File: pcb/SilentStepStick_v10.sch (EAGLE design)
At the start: 30 parts, among them X1 PASSER-07, X2 PASSER-07

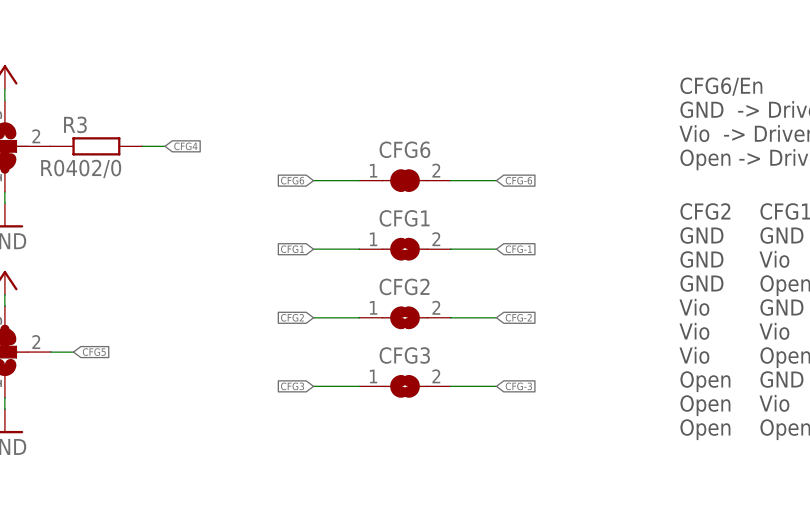
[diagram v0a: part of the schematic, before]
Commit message: updated layout and schematics
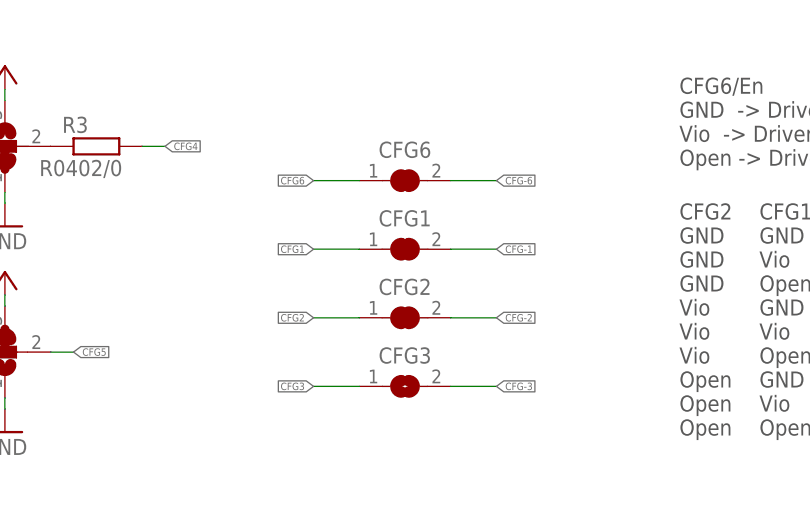
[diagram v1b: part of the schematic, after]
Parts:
- CFG1, CFG2, CFG3, CFG6: value JUMPER2-0201-NC -> JUMPER2-0201; device we-rcl:JUMPER2-0201-NC -> we-rcl:JUMPER2-0201
- CFG5: value JUMPER3-0201-NC -> JUMPER3-0201; device we-rcl:JUMPER3-0201-NC -> we-rcl:JUMPER3-0201
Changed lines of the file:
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@@
 <setting verticaltext="up"/>
 </settings>
-<grid distance="0.05" unitdist="inch" unit="inch" style="lines" multiple="1" display="yes" altdistance="0.025" altunitdist="inch" altunit="inch"/>
+<grid distance="0.1" unitdist="inch" unit="inch" style="lines" multiple="1" display="no" altdistance="0.01" altunitdist="inch" altunit="inch"/>
 <layers>
-<layer number="1" name="Top" color="4" fill="1" visible="no" active="no"/>
-<layer number="2" name="Route2" color="11" fill="1" visible="no" active="no"/>
-<layer number="3" name="Route3" color="4" fill="3" visible="no" active="no"/>
-<layer number="4" name="Route4" color="1" fill="4" visible="no" active="no"/>
-<layer number="5" name="Route5" color="4" fill="4" visible="no" active="no"/>
-<layer number="6" name="Route6" color="1" fill="8" visible="no" active="no"/>
-<layer number="7" name="Route7" color="4" fill="8" visible="no" active="no"/>
-<layer number="8" name="Route8" color="1" fill="2" visible="no" active="no"/>
-<layer number="9" name="Route9" color="4" fill="2" visible="no" active="no"/>
-<layer number="10" name="Route10" color="1" fill="7" visible="no" active="no"/>
-<layer number="11" name="Route11" color="4" fill="7" visible="no" active="no"/>
-<layer number="12" name="Route12" color="1" fill="5" visible="no" active="no"/>
-<layer number="13" name="Route13" color="4" fill="5" visible="no" active="no"/>
-<layer number="14" name="Route14" color="1" fill="6" visible="no" active="no"/>
-<layer number="15" name="Route15" color="13" fill="1" visible="no" active="no"/>
-<layer number="16" name="Bottom" color="1" fill="1" visible="no" active="no"/>
-<layer number="17" name="Pads" color="2" fill="1" visible="no" active="no"/>
-<layer number="18" name="Vias" color="2" fill="1" visible="no" active="no"/>
-<layer number="19" name="Unrouted" color="14" fill="1" visible="no" active="no"/>
-<layer number="20" name="Dimension" color="15" fill="1" visible="no" active="no"/>
-<layer number="21" name="tPlace" color="7" fill="1" visible="no" active="no"/>
-<layer number="22" name="bPlace" color="7" fill="1" visible="no" active="no"/>
-<layer number="23" name="tOrigins" color="15" fill="1" visible="no" active="no"/>
-<layer number="24" name="bOrigins" color="15" fill="1" visible="no" active="no"/>
-<layer number="25" name="tNames" color="7" fill="1" visible="no" active="no"/>
-<layer number="26" name="bNames" color="7" fill="1" visible="no" active="no"/>
-<layer number="27" name="tValues" color="7" fill="1" visible="no" active="no"/>
-<layer number="28" name="bValues" color="7" fill="1" visible="no" active="no"/>
+<layer number="1" name="Top" color="4" fill="1" visible="yes" active="no"/>
+<layer number="2" name="Route2" color="11" fill="1" visible="yes" active="no"/>
+<layer number="3" name="Route3" color="4" fill="3" visible="yes" active="no"/>
+<layer number="4" name="Route4" color="1" fill="4" visible="yes" active="no"/>
+<layer number="5" name="Route5" color="4" fill="4" visible="yes" active="no"/>
+<layer number="6" name="Route6" color="1" fill="8" visible="yes" active="no"/>
+<layer number="7" name="Route7" color="4" fill="8" visible="yes" active="no"/>
+<layer number="8" name="Route8" color="1" fill="2" visible="yes" active="no"/>
+<layer number="9" name="Route9" color="4" fill="2" visible="yes" active="no"/>
+<layer number="10" name="Route10" color="1" fill="7" visible="yes" active="no"/>
+<layer number="11" name="Route11" color="4" fill="7" visible="yes" active="no"/>
+<layer number="12" name="Route12" color="1" fill="5" visible="yes" active="no"/>
+<layer number="13" name="Route13" color="4" fill="5" visible="yes" active="no"/>
+<layer number="14" name="Route14" color="1" fill="6" visible="yes" active="no"/>
+<layer number="15" name="Route15" color="13" fill="1" visible="yes" active="no"/>
+<layer number="16" name="Bottom" color="1" fill="1" visible="yes" active="no"/>
+<layer number="17" name="Pads" color="2" fill="1" visible="yes" active="no"/>
+<layer number="18" name="Vias" color="2" fill="1" visible="yes" active="no"/>
+<layer number="19" name="Unrouted" color="14" fill="1" visible="yes" active="no"/>
+<layer number="20" name="Dimension" color="15" fill="1" visible="yes" active="no"/>
+<layer number="21" name="tPlace" color="7" fill="1" visible="yes" active="no"/>
+<layer number="22" name="bPlace" color="7" fill="1" visible="yes" active="no"/>
+<layer number="23" name="tOrigins" color="15" fill="1" visible="yes" active="no"/>
+<layer number="24" name="bOrigins" color="15" fill="1" visible="yes" active="no"/>
+<layer number="25" name="tNames" color="7" fill="1" visible="yes" active="no"/>
+<layer number="26" name="bNames" color="7" fill="1" visible="yes" active="no"/>
+<layer number="27" name="tValues" color="7" fill="1" visible="yes" active="no"/>
+<layer number="28" name="bValues" color="7" fill="1" visible="yes" active="no"/>
 <layer number="29" name="tStop" color="7" fill="3" visible="no" active="no"/>
 <layer number="30" name="bStop" color="7" fill="6" visible="no" active="no"/>
@@
 <layer number="35" name="tGlue" color="7" fill="4" visible="no" active="no"/>
 <layer number="36" name="bGlue" color="7" fill="5" visible="no" active="no"/>
-<layer number="37" name="tTest" color="7" fill="1" visible="no" active="no"/>
-<layer number="38" name="bTest" color="7" fill="1" visible="no" active="no"/>
+<layer number="37" name="tTest" color="7" fill="1" visible="yes" active="no"/>
+<layer number="38" name="bTest" color="7" fill="1" visible="yes" active="no"/>
 <layer number="39" name="tKeepout" color="4" fill="11" visible="no" active="no"/>
 <layer number="40" name="bKeepout" color="1" fill="11" visible="no" active="no"/>
@@
 <layer number="44" name="Drills" color="7" fill="1" visible="no" active="no"/>
 <layer number="45" name="Holes" color="7" fill="1" visible="no" active="no"/>
-<layer number="46" name="Milling" color="3" fill="1" visible="no" active="no"/>
-<layer number="47" name="Measures" color="7" fill="1" visible="no" active="no"/>
-<layer number="48" name="Document" color="7" fill="1" visible="no" active="no"/>
-<layer number="49" name="Reference" color="7" fill="1" visible="no" active="no"/>
-<layer number="50" name="dxf" color="7" fill="1" visible="no" active="no"/>
-<layer number="51" name="tDocu" color="7" fill="1" visible="no" active="no"/>
-<layer number="52" name="bDocu" color="7" fill="1" visible="no" active="no"/>
-<layer number="53" name="tPadExt" color="7" fill="6" visible="no" active="no"/>
-<layer number="54" name="bPadExt" color="1" fill="3" visible="no" active="no"/>
-<layer number="56" name="wert" color="7" fill="1" visible="no" active="no"/>
-<layer number="57" name="tCAD" color="7" fill="1" visible="no" active="no"/>
+<layer number="46" name="Milling" color="3" fill="1" visible="yes" active="no"/>
+<layer number="47" name="Measures" color="7" fill="1" visible="yes" active="no"/>
+<layer number="48" name="Document" color="7" fill="1" visible="yes" active="no"/>
+<layer number="49" name="Reference" color="7" fill="1" visible="yes" active="no"/>
+<layer number="50" name="dxf" color="7" fill="1" visible="yes" active="no"/>
+<layer number="51" name="tDocu" color="7" fill="1" visible="yes" active="no"/>
+<layer number="52" name="bDocu" color="7" fill="1" visible="yes" active="no"/>
+<layer number="53" name="tPadExt" color="7" fill="6" visible="yes" active="no"/>
+<layer number="54" name="bPadExt" color="1" fill="3" visible="yes" active="no"/>
+<layer number="56" name="wert" color="7" fill="1" visible="yes" active="no"/>
+<layer number="57" name="tCAD" color="7" fill="1" visible="yes" active="no"/>
 <layer number="91" name="Nets" color="2" fill="1" visible="yes" active="yes"/>
 <layer number="92" name="Busses" color="1" fill="1" visible="yes" active="yes"/>
@@
 <part name="GND15" library="supply1" deviceset="GND" device=""/>
 <part name="P+3" library="supply1" deviceset="+5V" device=""/>
-<part name="CFG3" library="we-rcl" deviceset="JUMPER2" device="-0201-NC"/>
+<part name="CFG3" library="we-rcl" deviceset="JUMPER2" device="-0201" value="JUMPER2-0201"/>
 <part name="CFG4" library="we-rcl" deviceset="JUMPER3" device="-0201-NC"/>
-<part name="CFG5" library="we-rcl" deviceset="JUMPER3" device="-0201-NC"/>
-<part name="CFG6" library="we-rcl" deviceset="JUMPER2" device="-0201-NC"/>
-<part name="CFG1" library="we-rcl" deviceset="JUMPER2" device="-0201-NC"/>
-<part name="CFG2" library="we-rcl" deviceset="JUMPER2" device="-0201-NC"/>
+<part name="CFG5" library="we-rcl" deviceset="JUMPER3" device="-0201" value="JUMPER3-0201"/>
+<part name="CFG6" library="we-rcl" deviceset="JUMPER2" device="-0201" value="JUMPER2-0201"/>
+<part name="CFG1" library="we-rcl" deviceset="JUMPER2" device="-0201" value="JUMPER2-0201"/>
+<part name="CFG2" library="we-rcl" deviceset="JUMPER2" device="-0201" value="JUMPER2-0201"/>
 <part name="R3" library="rcl" deviceset="R-EU_" device="R0402" value="R0402/0"/>
 <part name="R6" library="we-rcl" deviceset="POT" device="EVM3R"/>
@@
 stealthChop
 stealthChop</text>
+<wire x1="59.055" y1="31.75" x2="60.325" y2="31.75" width="1.016" layer="94"/>
+<wire x1="59.055" y1="24.13" x2="60.325" y2="24.13" width="1.016" layer="94"/>
 </plain>
 <instances>
